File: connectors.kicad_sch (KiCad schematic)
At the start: 10 parts, among them J10 SM02B-SRSS-TB(LF)(SN), J11 SM02B-SRSS-TB(LF)(SN), J6 SM04B-SRSS-TB(LF)(SN), J7 SM04B-SRSS-TB(LF)(SN), J8 SM04B-SRSS-TB(LF)(SN), J9 SM04B-SRSS-TB(LF)(SN)

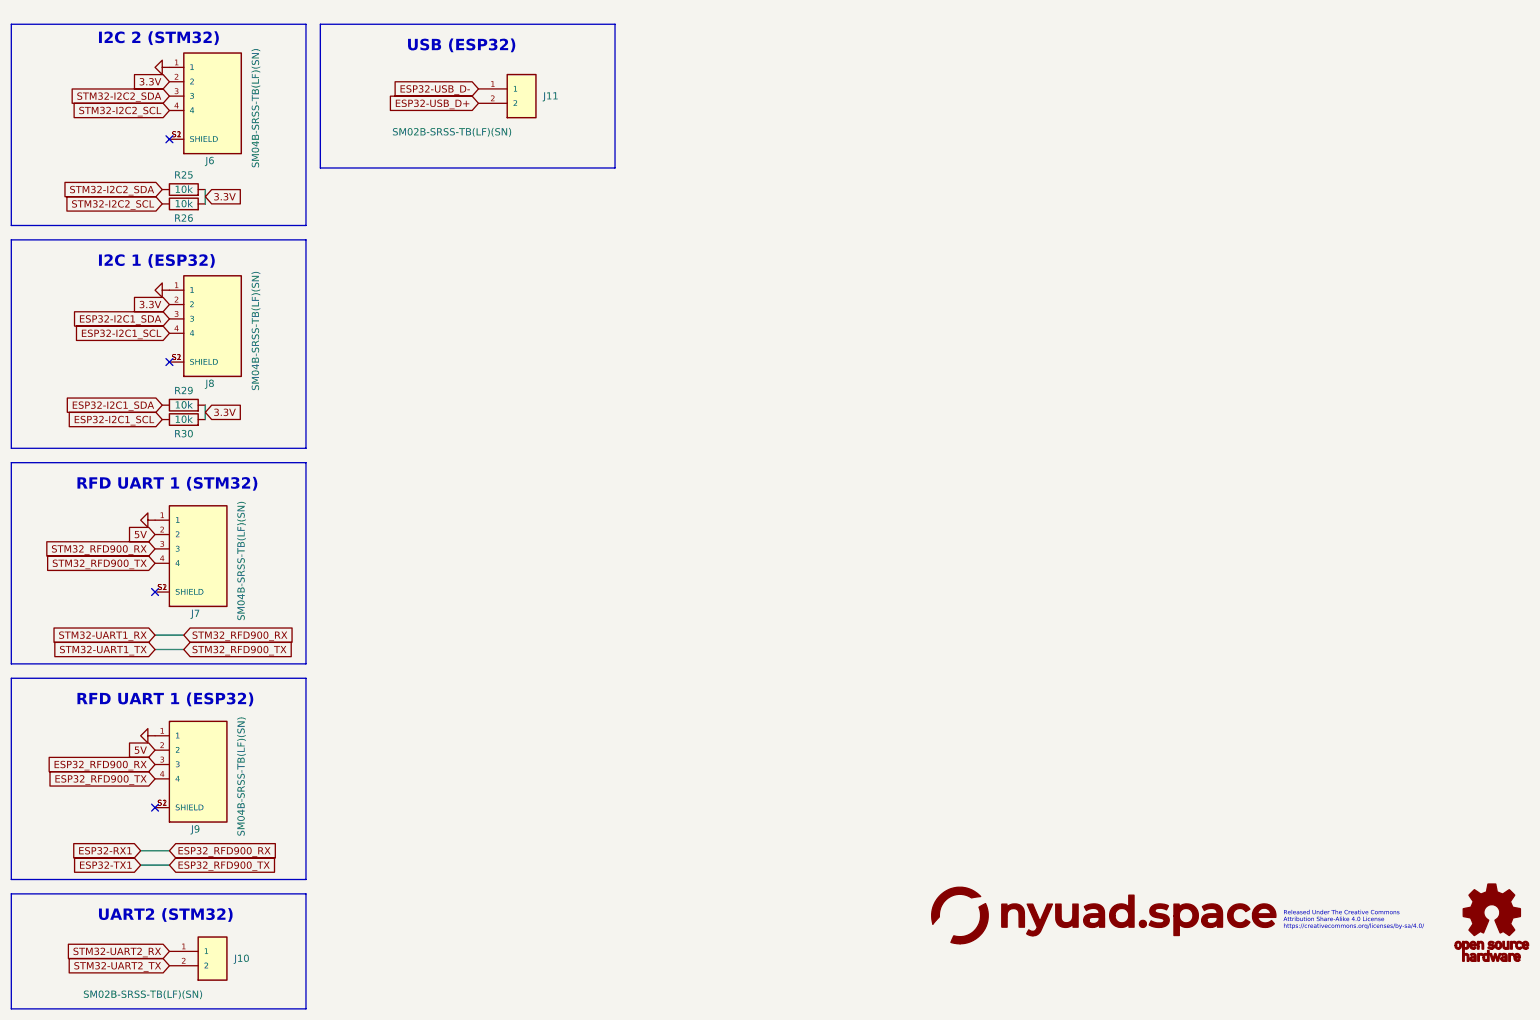
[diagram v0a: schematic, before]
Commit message: Updated files
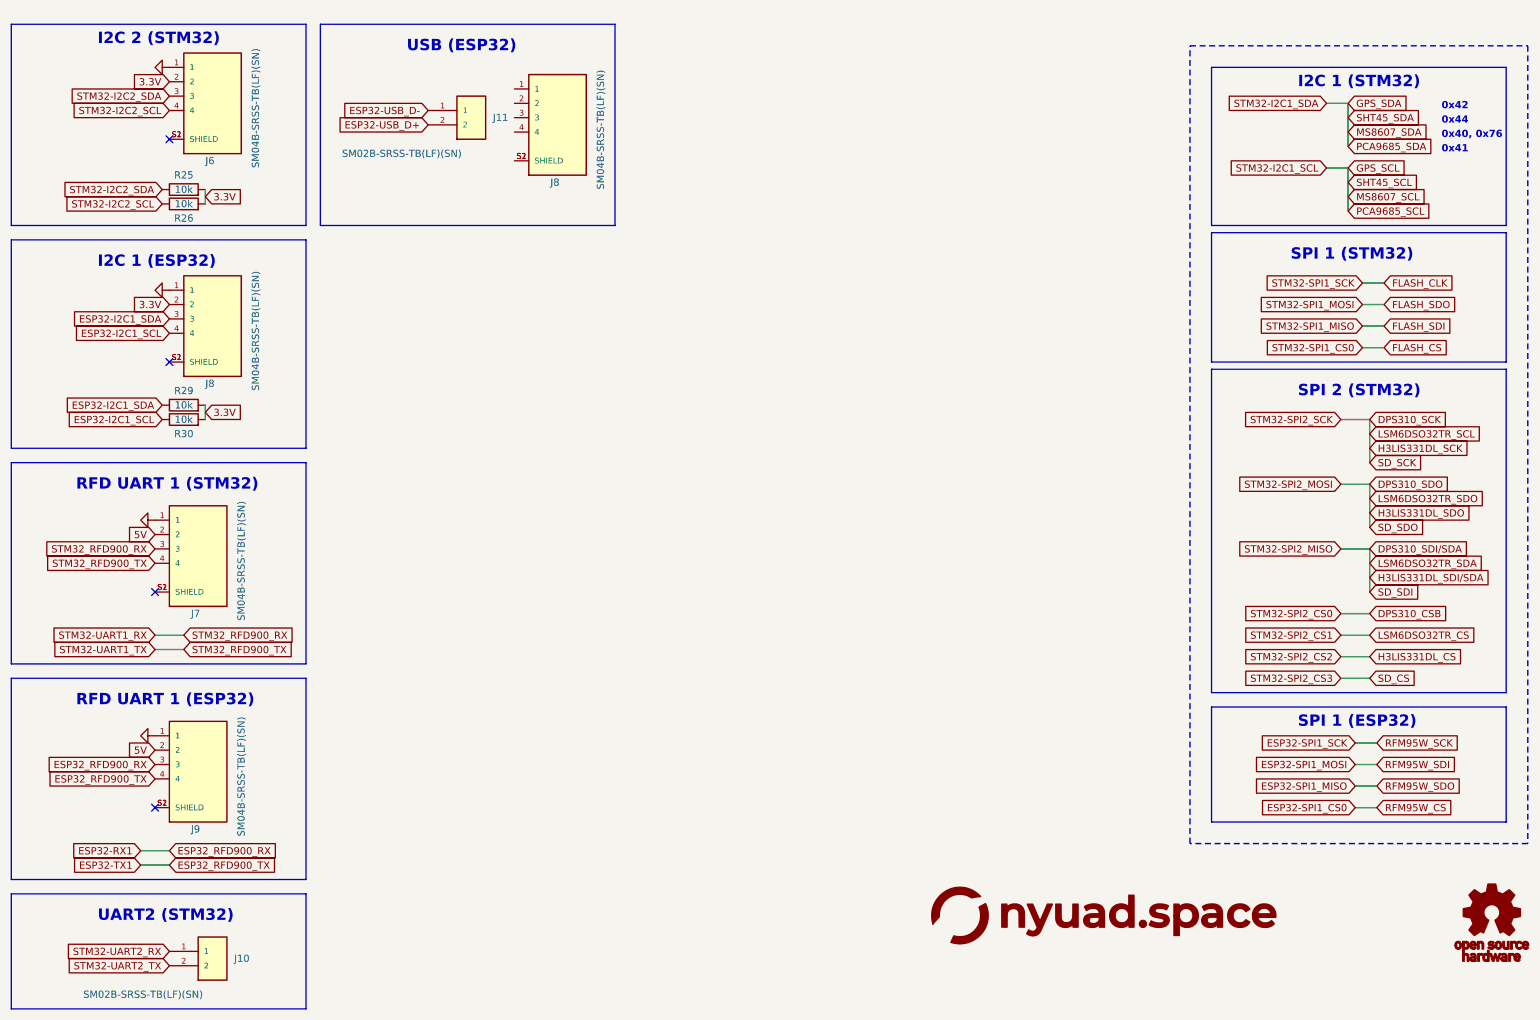
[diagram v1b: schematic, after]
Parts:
- added J8: SM04B-SRSS-TB(LF)(SN), JST_SM04B-SRSS-TB(LF)(SN), symbol SM04B-SRSS-TB_LF__SN_:SM04B-SRSS-TB(LF)(SN)
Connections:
- new net: J8.S1 (SHIELD), J8.S2 (SHIELD)
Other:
- note added: "0x40, 0x76"
- note added: "0x41"
- note added: "0x42"
- note added: "0x44"
- note added: "I2C 1 (STM32)"
- note added: "SPI 1 (ESP32)"
- note added: "SPI 1 (STM32)"
- note added: "SPI 2 (STM32)"
- note removed: "Released Under The Creative Commons Attribution Share-Alike 4.0 License https://creativecommons.orq/licenses/by-sa/4.0/"
- title: Connectors & Peripherals -> Connections & Peripherals
- moved on the sheet: J11
